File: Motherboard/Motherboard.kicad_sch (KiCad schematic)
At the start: 53 parts, among them J1 40-pin IDE Connector, J3 Bus_ISA_8bit, J4 ATX-24, J5 USB_B, J6 ATF15XX_JTAG_ISP, J7 Bus_ISA_8bit, J8 65SIB_Connector, SW1 SW_Push, SW2 SW_SPST, U1 AS6C8008, U10 ATF1508AS-PLCC84, U11 74HCT245, U12 74HCT573, U13 8255, U14 WD65C22, U15 AS6C8008, U16 MCP2200-I-SO, U17 74HCT163, U18 LM7905_TO220, U19 GAL16V8, U2 74HCT04, U3 SC28L91, U4 SST39SF040, U5 SST39SF040, U6 SST39SF040, U7 SST39SF040, U8 WD65C816S, U9 DS1813, X1 ACO-3.6864MHz, X2 ACO-24MHz, X3 ACO-14.31818MHz

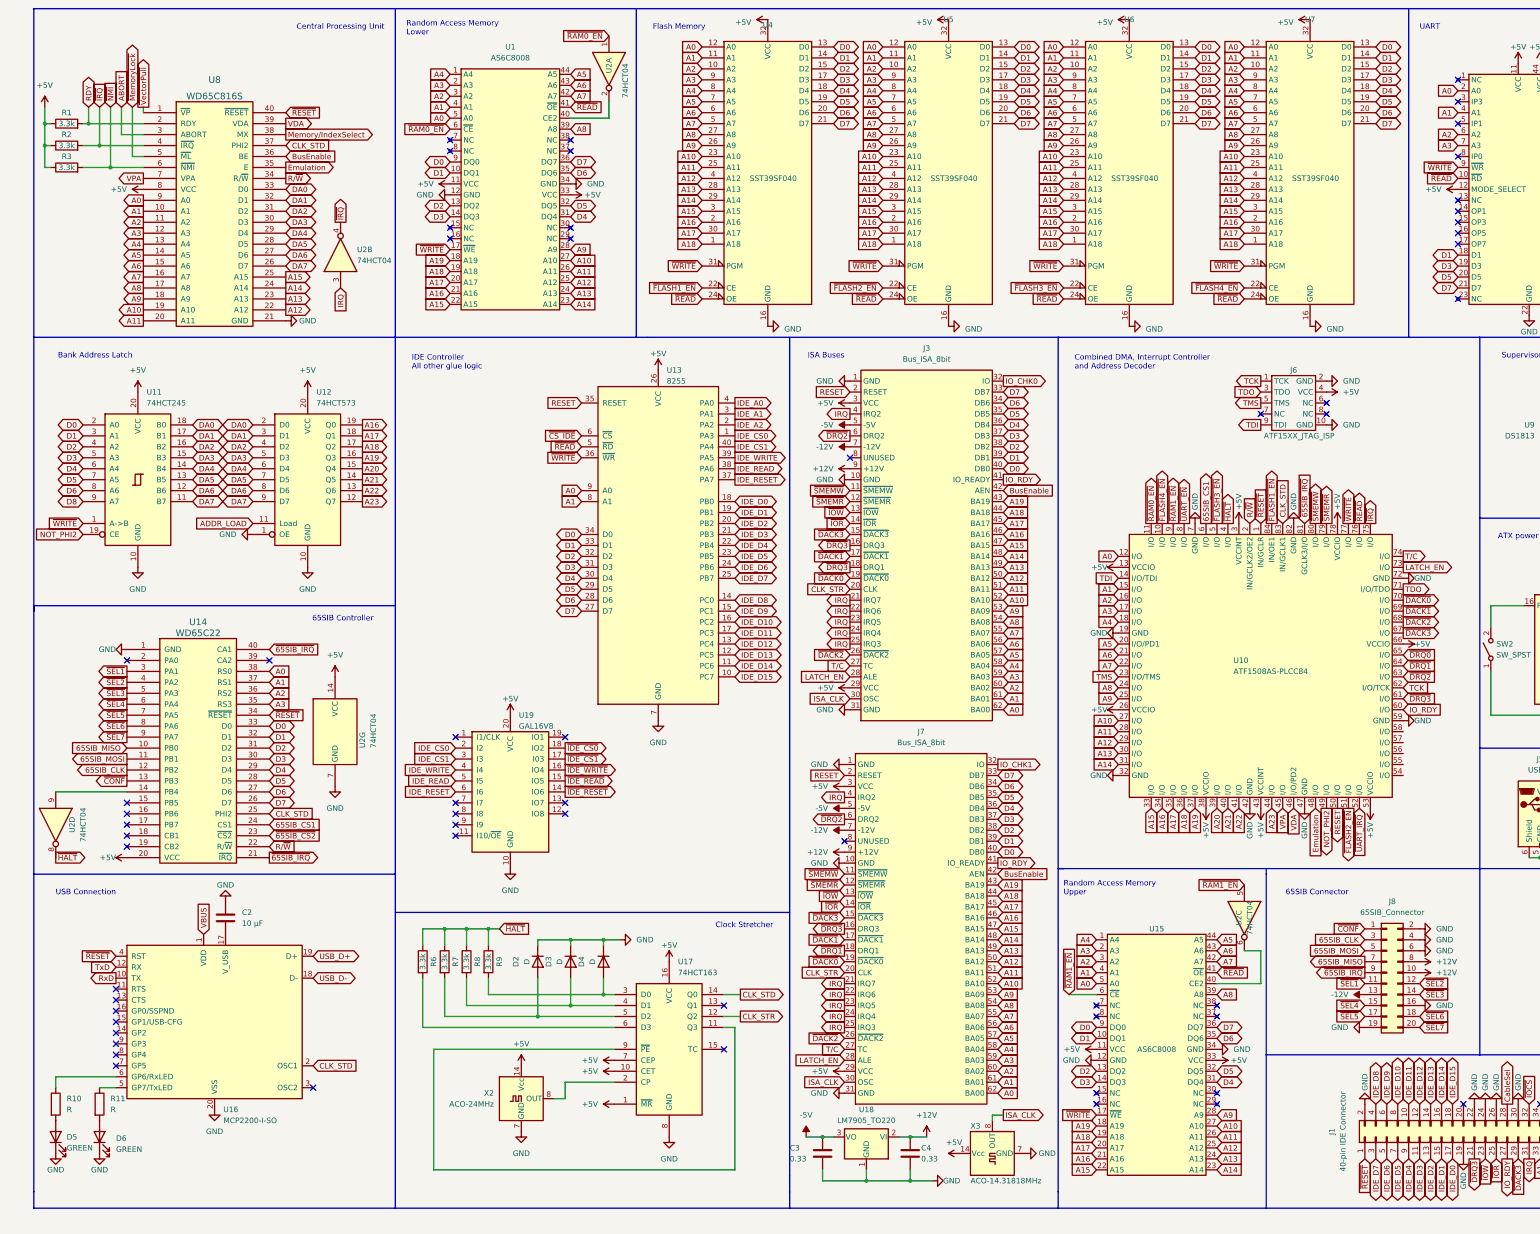
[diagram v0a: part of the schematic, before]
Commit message: Fixed clock connections...
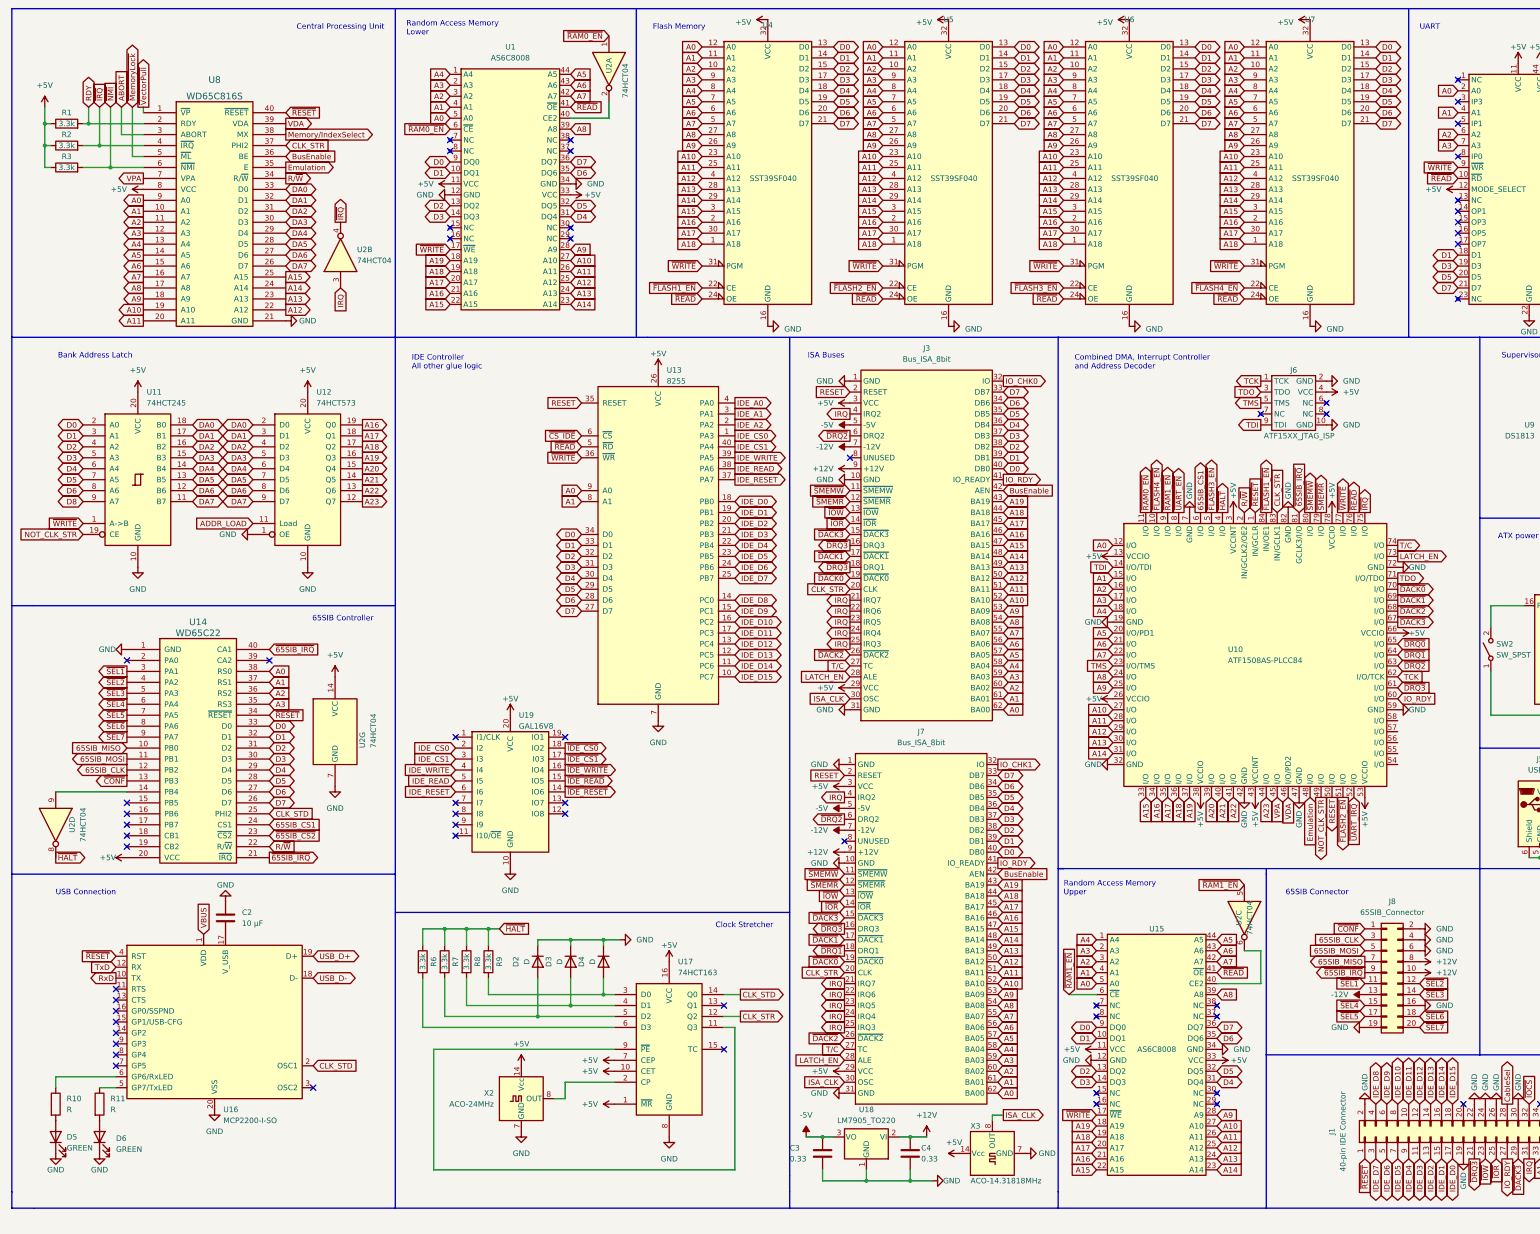
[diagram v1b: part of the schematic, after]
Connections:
- net CLK_STD: no longer U10.83 (IN/GCLK1), U8.37 (PHI2)
- net CLK_STR: now also U10.83 (IN/GCLK1), U8.37 (PHI2)
- net NOT_PHI2 renamed NOT_CLK_STR
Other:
- moved on the sheet: U10
